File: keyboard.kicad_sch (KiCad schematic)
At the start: 88 parts, among them SW1 SW_PUSH, SW10 SW_PUSH, SW11 SW_PUSH, SW12 SW_PUSH, SW13 SW_PUSH, SW14 SW_PUSH, SW15 SW_PUSH, SW16 SW_PUSH, SW17 SW_PUSH, SW18 SW_PUSH, SW19 SW_PUSH, SW2 SW_PUSH, SW20 SW_PUSH, SW21 SW_PUSH, SW22 SW_PUSH, SW23 SW_PUSH, SW24 SW_PUSH, SW25 SW_PUSH, SW26 SW_PUSH, SW27 SW_PUSH, SW28 SW_PUSH, SW29 SW_PUSH, SW3 SW_PUSH, SW30 SW_PUSH, SW31 SW_PUSH, SW32 SW_PUSH, SW33 SW_PUSH, SW34 SW_PUSH, SW35 SW_PUSH, SW36 SW_PUSH, SW37 SW_PUSH, SW38 SW_PUSH, SW39 SW_PUSH, SW4 SW_PUSH, SW40 SW_PUSH, SW41 SW_PUSH, SW42 SW_PUSH, SW43 SW_PUSH, SW5 SW_PUSH, SW6 SW_PUSH, SW7 SW_PUSH, SW8 SW_PUSH, SW9 SW_PUSH, U1 Pico

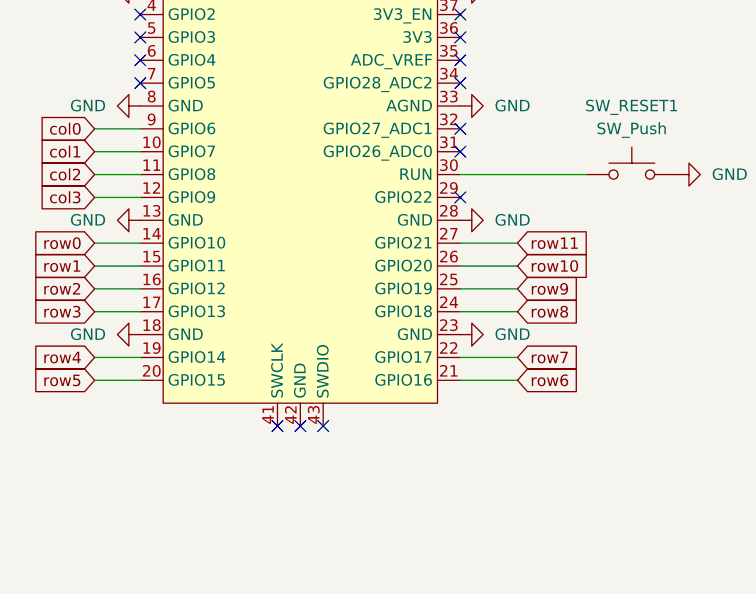
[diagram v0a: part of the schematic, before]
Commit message: :construction:
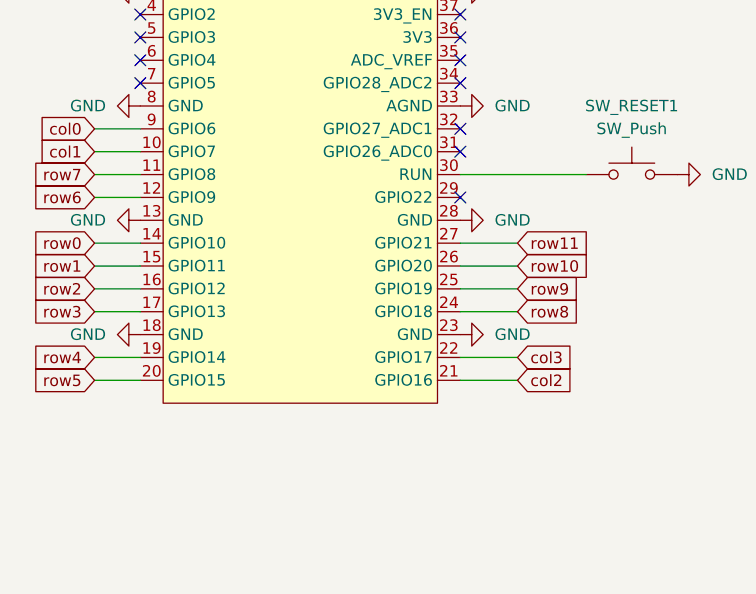
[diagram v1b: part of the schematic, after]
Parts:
- D1, D10, D11, D12, D13, D14, D15, D16, D17, D18, D19, D2, D20, D21, D22, D23, D24, D25, D26, D27, D28, D29, D3, D30, D31, D32, D33, D34, D35, D36, D37, D38, D39, D4, D40, D41, D42, D43, D5, D6, D7, D8, D9: footprint kbd:D3_SMD_v2 -> Diode_SMD:D_SOD-123
- U1: symbol MCU_RaspberryPi_and_Boards:Pico -> mikamo3:Raspberry_Pi_Pico(without_debugPin)
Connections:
- net col2: now also U1.21 (GPIO16); no longer U1.11 (GPIO8)
- net col3: now also U1.22 (GPIO17); no longer U1.12 (GPIO9)
- net row6: now also U1.12 (GPIO9); no longer U1.21 (GPIO16)
- net row7: now also U1.11 (GPIO8); no longer U1.22 (GPIO17)
- no-connect marks 17 -> 14

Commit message: :construction:
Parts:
- added D44, D45, D46, D47, D48, D49: D, Diode_SMD:D_SOD-123, symbol Device:D
- added SW44, SW45, SW46, SW47: SW_PUSH, mikamo3:CherryMX_Hotswap_1u, symbol kbd:SW_PUSH
- added SW48, SW49: RotaryEncoder_Switch, Rotary_Encoder:RotaryEncoder_Alps_EC12E-Switch_Vertical_H20mm, symbol Device:RotaryEncoder_Switch
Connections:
- net GND: now also SW48.C, SW49.C
- net row0: now also SW44.1
- net row1: now also SW45.1
- net row2: now also SW46.1
- net row3: now also SW47.1
- net row4: now also SW48.S2
- net row5: now also SW49.S2
- net enc_0_a: now reaches U1.29 (GPIO22)
- net enc_0_a: now also SW48.A
- net enc_0_b: now reaches U1.31 (GPIO26_ADC0)
- net enc_0_b: now also SW48.B
- net enc_1_a: now reaches U1.32 (GPIO27_ADC1)
- net enc_1_a: now also SW49.A
- net enc_1_b: now reaches U1.34 (GPIO28_ADC2)
- net enc_1_b: now also SW49.B
- net col4: now reaches U1.7 (GPIO5)
- net col4: now also D44.1 (K), D45.1 (K), D46.1 (K), D47.1 (K), D48.1 (K), D49.1 (K)
- new net: D45.2 (A), SW45.2
- new net: D44.2 (A), SW44.2
- new net: D49.2 (A), SW49.S1
- new net: D46.2 (A), SW46.2
- new net: D47.2 (A), SW47.2
- new net: D48.2 (A), SW48.S1
- no-connect marks 14 -> 9
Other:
- moved on the sheet: D1, D10, D11, D12, D13, D14, D15, D16, D17, D18, D19, D2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
